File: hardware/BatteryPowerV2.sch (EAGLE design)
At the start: 66 parts, among them Q1 IRLML6402, U1 LT1616ES6TRMPBF, U2 LT6106CS5#PBF, U3 LT1616ES6TRMPBF, U4 LT6106CS5#PBF, U5 TCK106AF,LF, U6 TCK106AF,LF

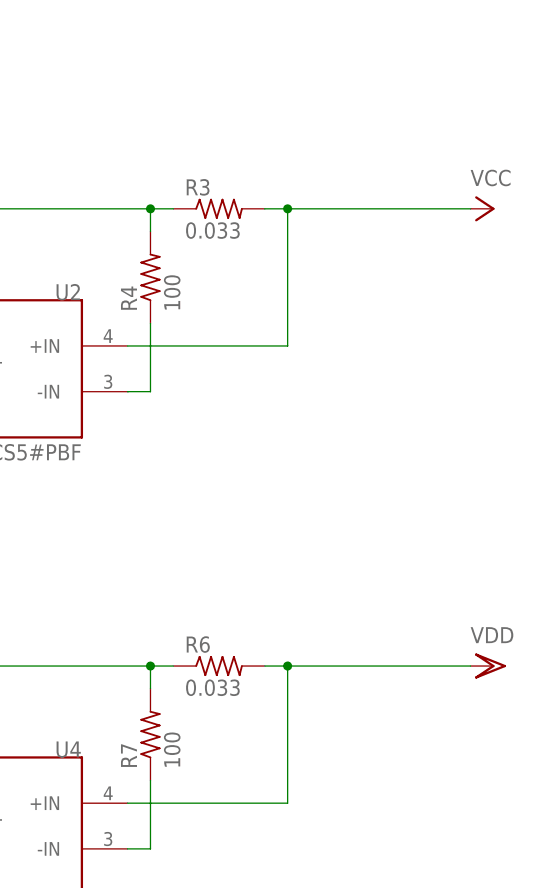
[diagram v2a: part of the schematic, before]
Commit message: 微調整
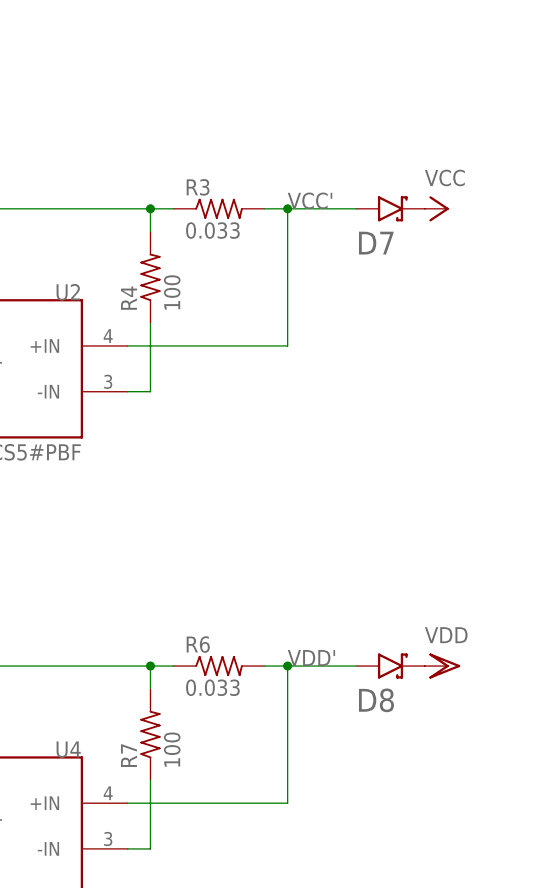
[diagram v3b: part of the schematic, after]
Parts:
- added D7, D8: CUHS20S30, diodes:CUHS20S30
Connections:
- new net VCC': D7.A, R3.2, U2.+IN
- new net VDD': D8.A, R6.2, U4.+IN
- net VCC: now also D7.C; no longer R3.2, U2.+IN
- net VDD: now also D8.C; no longer R6.2, U4.+IN
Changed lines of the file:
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@@
 <part name="R21" library="rcl" library_urn="urn:adsk.eagle:library:334" deviceset="R-US_" device="R0603" package3d_urn="urn:adsk.eagle:package:23555/3" value="100k"/>
 <part name="GND31" library="supply1" library_urn="urn:adsk.eagle:library:371" deviceset="GND" device=""/>
+<part name="D7" library="diodes" deviceset="CUHS20S30" device=""/>
+<part name="D8" library="diodes" deviceset="CUHS20S30" device=""/>
 </parts>
 <sheets>
@@
 <attribute name="VALUE" x="335.28" y="88.9" size="1.778" layer="96" rot="R180"/>
 </instance>
-<instance part="P+1" gate="VCC" x="441.96" y="101.6" smashed="yes" rot="R270">
-<attribute name="VALUE" x="439.42" y="104.14" size="1.778" layer="96"/>
+<instance part="P+1" gate="VCC" x="436.88" y="101.6" smashed="yes" rot="R270">
+<attribute name="VALUE" x="434.34" y="104.14" size="1.778" layer="96"/>
 </instance>
 <instance part="U3" gate="A" x="320.04" y="38.1" smashed="yes" rot="MR0">
@@
 <attribute name="VALUE" x="335.28" y="38.1" size="1.778" layer="96" rot="R180"/>
 </instance>
-<instance part="VDD1" gate="G$1" x="441.96" y="50.8" smashed="yes" rot="R270">
-<attribute name="VALUE" x="439.42" y="53.34" size="1.778" layer="96"/>
+<instance part="VDD1" gate="G$1" x="436.88" y="50.8" smashed="yes" rot="R270">
+<attribute name="VALUE" x="434.34" y="53.34" size="1.778" layer="96"/>
 </instance>
 <instance part="C5" gate="G$1" x="251.46" y="27.94" smashed="yes">
@@
 <instance part="GND31" gate="1" x="210.82" y="68.58" smashed="yes">
 <attribute name="VALUE" x="208.28" y="66.04" size="1.778" layer="96"/>
+</instance>
+<instance part="D7" gate="G$1" x="431.8" y="101.6" smashed="yes">
+<attribute name="NAME" x="426.72" y="96.52" size="2.54" layer="95"/>
+</instance>
+<instance part="D8" gate="G$1" x="431.8" y="50.8" smashed="yes">
+<attribute name="NAME" x="426.72" y="45.72" size="2.54" layer="95"/>
 </instance>
 </instances>
@@
 </segment>
 <segment>
-<pinref part="R3" gate="G$1" pin="2"/>
-<wire x1="416.56" y1="101.6" x2="419.1" y2="101.6" width="0.1524" layer="91"/>
-<wire x1="419.1" y1="101.6" x2="439.42" y2="101.6" width="0.1524" layer="91"/>
-<pinref part="U2" gate="G$1" pin="+IN"/>
-<wire x1="401.32" y1="86.36" x2="419.1" y2="86.36" width="0.1524" layer="91"/>
-<wire x1="419.1" y1="86.36" x2="419.1" y2="101.6" width="0.1524" layer="91"/>
-<junction x="419.1" y="101.6"/>
-<pinref part="P+1" gate="VCC" pin="VCC"/>
-</segment>
-<segment>
 <pinref part="U5" gate="G$1" pin="VIN"/>
 <wire x1="281.94" y1="-12.7" x2="279.4" y2="-12.7" width="0.1524" layer="91"/>
 <wire x1="279.4" y1="-12.7" x2="279.4" y2="-10.16" width="0.1524" layer="91"/>
 <pinref part="P+2" gate="VCC" pin="VCC"/>
+</segment>
+<segment>
+<pinref part="D7" gate="G$1" pin="C"/>
+<pinref part="P+1" gate="VCC" pin="VCC"/>
 </segment>
 </net>
@@
 </segment>
 <segment>
-<pinref part="R6" gate="G$1" pin="2"/>
-<wire x1="416.56" y1="50.8" x2="419.1" y2="50.8" width="0.1524" layer="91"/>
-<wire x1="419.1" y1="50.8" x2="439.42" y2="50.8" width="0.1524" layer="91"/>
-<pinref part="U4" gate="G$1" pin="+IN"/>
-<wire x1="401.32" y1="35.56" x2="419.1" y2="35.56" width="0.1524" layer="91"/>
-<wire x1="419.1" y1="35.56" x2="419.1" y2="50.8" width="0.1524" layer="91"/>
-<junction x="419.1" y="50.8"/>
-<pinref part="VDD1" gate="G$1" pin="VDD"/>
-</segment>
-<segment>
 <pinref part="U6" gate="G$1" pin="VIN"/>
 <wire x1="281.94" y1="-33.02" x2="279.4" y2="-33.02" width="0.1524" layer="91"/>
@@
 <pinref part="VDD3" gate="G$1" pin="VDD"/>
 <wire x1="355.6" y1="139.7" x2="355.6" y2="144.78" width="0.1524" layer="91"/>
+</segment>
+<segment>
+<pinref part="D8" gate="G$1" pin="C"/>
+<pinref part="VDD1" gate="G$1" pin="VDD"/>
 </segment>
 </net>
@@
 </segment>
 </net>
+<net name="VDD'" class="0">
+<segment>
+<pinref part="R6" gate="G$1" pin="2"/>
+<wire x1="416.56" y1="50.8" x2="419.1" y2="50.8" width="0.1524" layer="91"/>
+<pinref part="U4" gate="G$1" pin="+IN"/>
+<wire x1="401.32" y1="35.56" x2="419.1" y2="35.56" width="0.1524" layer="91"/>
+<wire x1="419.1" y1="35.56" x2="419.1" y2="50.8" width="0.1524" layer="91"/>
+<wire x1="419.1" y1="50.8" x2="426.72" y2="50.8" width="0.1524" layer="91"/>
+<junction x="419.1" y="50.8"/>
+<pinref part="D8" gate="G$1" pin="A"/>
+<label x="419.1" y="50.8" size="1.778" layer="95"/>
+</segment>
+</net>
+<net name="VCC'" class="0">
+<segment>
+<pinref part="R3" gate="G$1" pin="2"/>
+<wire x1="416.56" y1="101.6" x2="419.1" y2="101.6" width="0.1524" layer="91"/>
+<pinref part="U2" gate="G$1" pin="+IN"/>
+<wire x1="401.32" y1="86.36" x2="419.1" y2="86.36" width="0.1524" layer="91"/>
+<wire x1="419.1" y1="86.36" x2="419.1" y2="101.6" width="0.1524" layer="91"/>
+<wire x1="419.1" y1="101.6" x2="426.72" y2="101.6" width="0.1524" layer="91"/>
+<junction x="419.1" y="101.6"/>
+<pinref part="D7" gate="G$1" pin="A"/>
+<label x="419.1" y="101.6" size="1.778" layer="95"/>
+</segment>
+</net>
